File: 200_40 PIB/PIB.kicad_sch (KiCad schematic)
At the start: 34 parts, among them J1 Igniter, J10 TC2, J2 Rogowski, J3 PIB Interface, J6 Main Disch, J7 Heater 1, J8 Heater 1, J9 TC1, Q1 3300V, Q3 VO3120, Q8 IRF7403, Q9 IRF7403, U1 ACS37042KLHBLT-030B3, U10 TLP3543, U11 STM32G431KBTx, U14 VO618A, U3 BDJ2FC0WEFJ

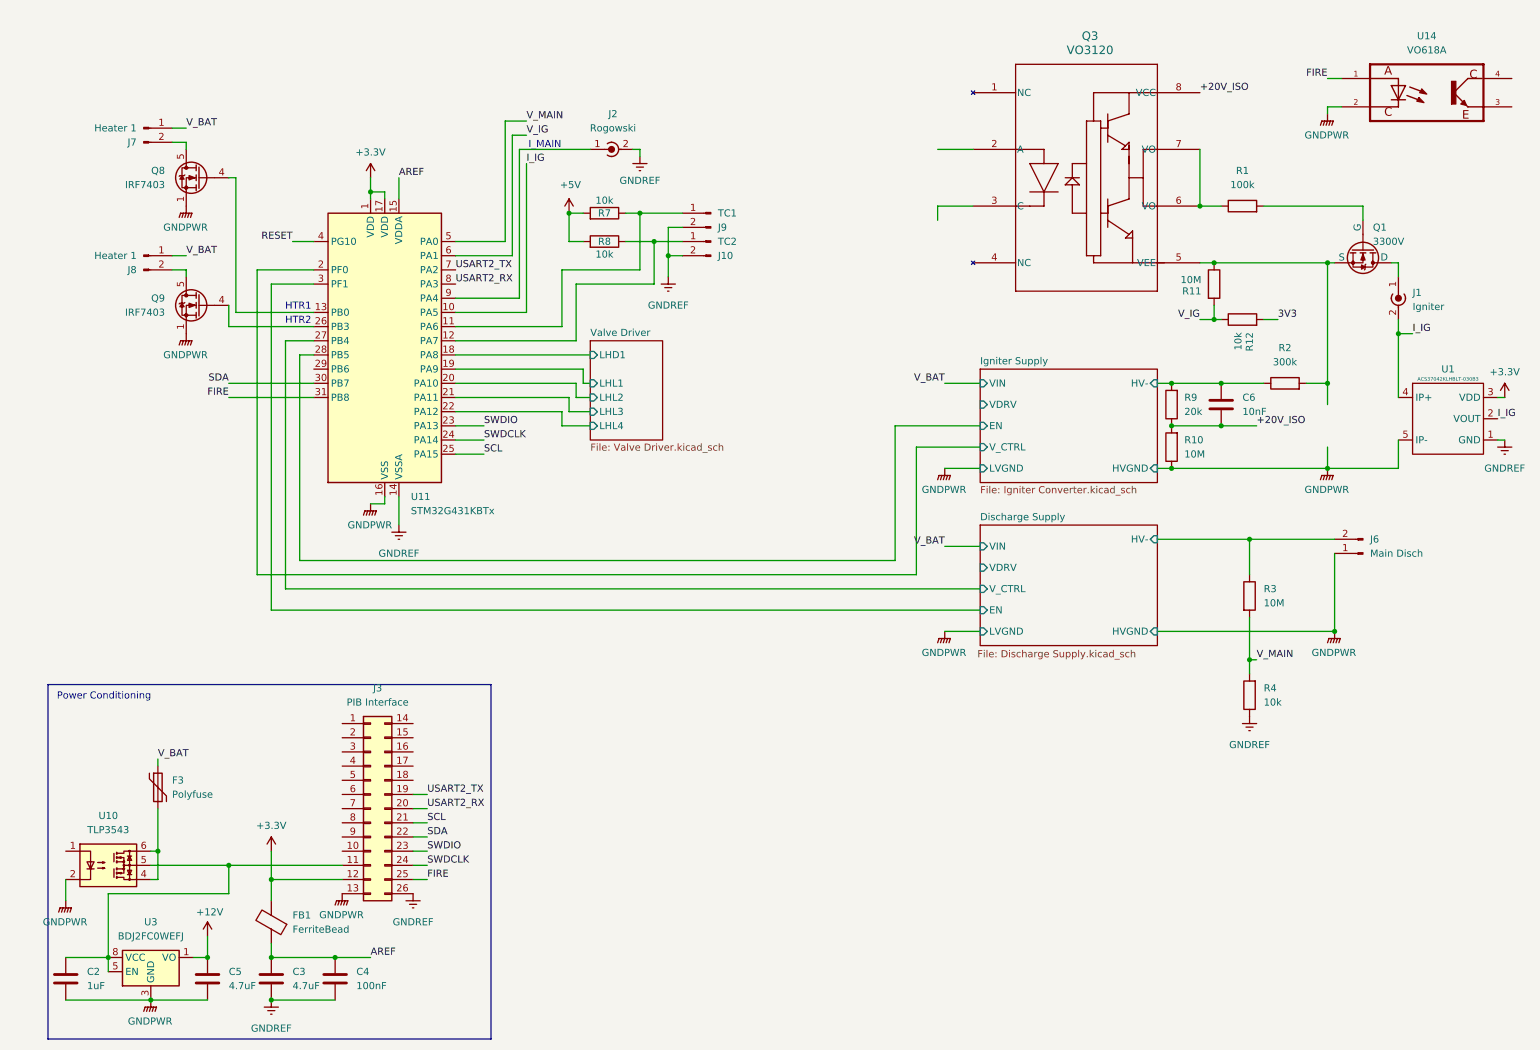
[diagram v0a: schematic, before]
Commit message: remove converters from PIB. WIP, do not check out
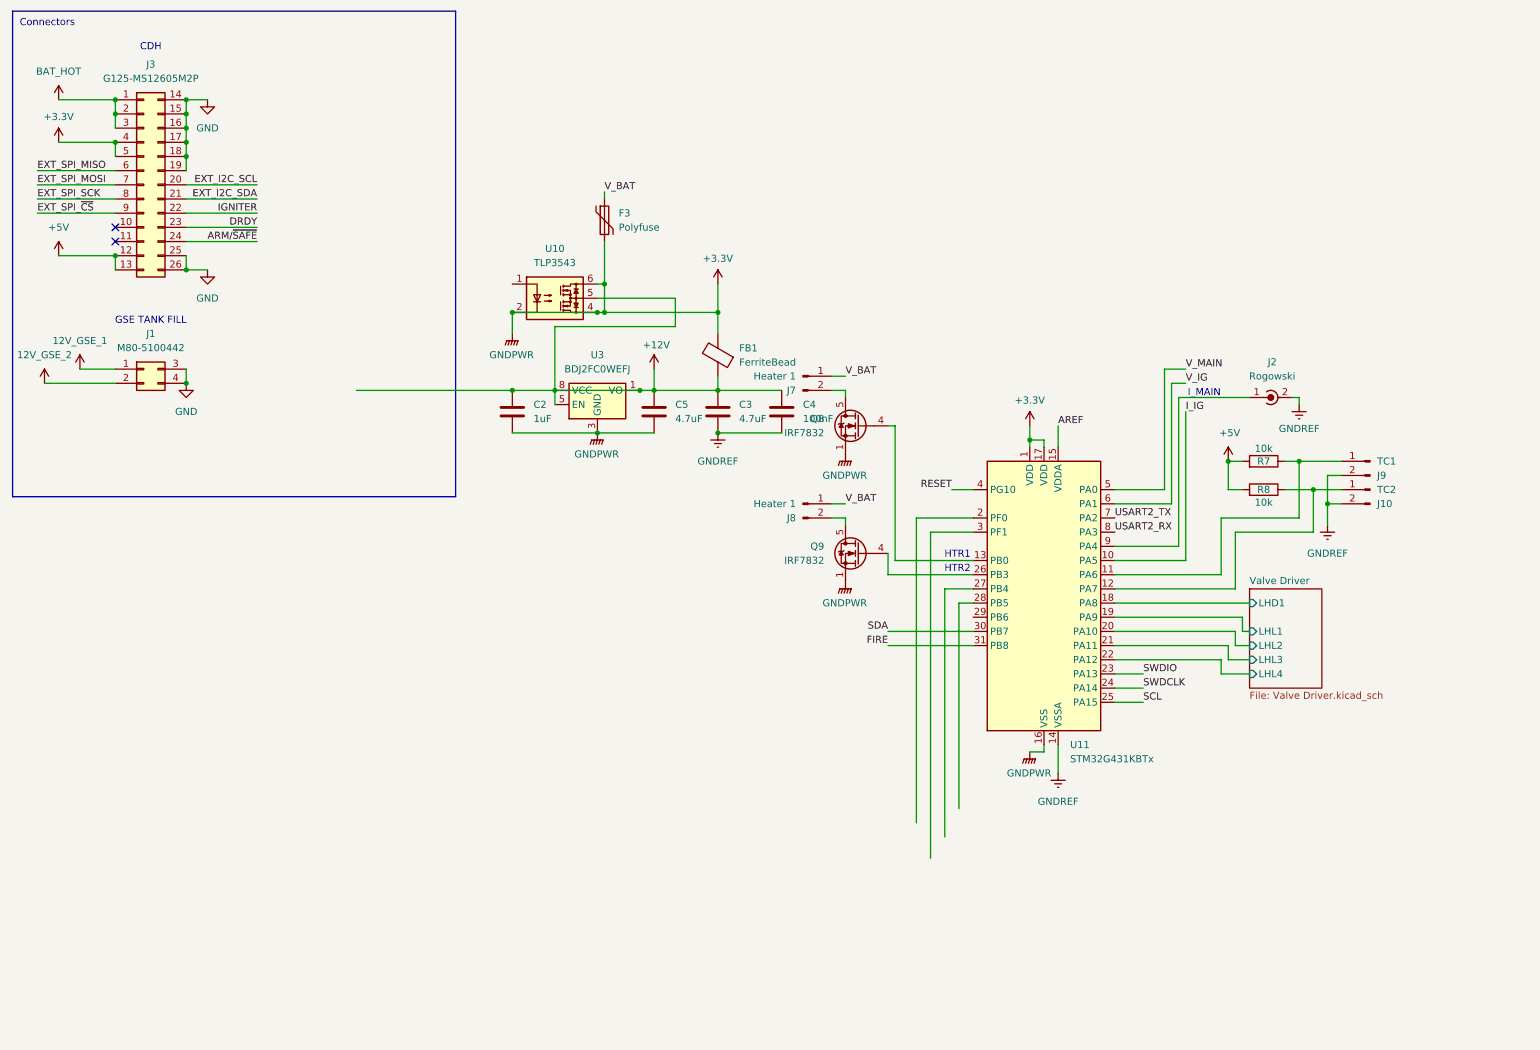
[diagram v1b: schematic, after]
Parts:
- removed C6: 10nF, symbol Device:C
- removed J1: Igniter, symbol Connector:Conn_Coaxial_Power
- removed J6: Main Disch, symbol Connector:Conn_01x02_Pin
- removed Q1: 3300V, Package_TO_SOT_THT:TO-247-4_Horizontal_TabDown, symbol Simulation_SPICE:NMOS
- removed Q3: VO3120, DIP_3120_VIS, symbol PIB_Symbol_Library:VO3120
- removed R1: 100k, symbol Device:R
- removed R10, R11, R3: 10M, symbol Device:R
- removed R12, R4: 10k, symbol Device:R
- removed R2: 300k, symbol Device:R
- removed R9: 20k, symbol Device:R
- removed U1: ACS37042KLHBLT-030B3, Package_TO_SOT_SMD:SOT-23-5_HandSoldering, symbol 0_PAY_Symbol_Library:ACS37042KLHBLT-030B3
- removed U14: VO618A, VO618A:DIP762W50P254L458H480Q4, symbol 0_PAY_Symbol_Library:VO618A
- added J1: M80-5100442, Package_LCC:PLCC-84_29.3x29.3mm_P1.27mm, symbol Connector_Generic:Conn_02x02_Top_Bottom
- J3: value PIB Interface -> G125-MS12605M2P
- Q8, Q9: value IRF7403 -> IRF7832
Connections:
- net +12V: now also C2.1, C3.1, C4.1, FB1.1, U10.5, U3.5 (EN), U3.8 (VCC)
- net +3.3V: now also C2.2, C5.2, F3.2, J3.4 (Pin_4), J3.5 (Pin_5), Q8.1 (S), Q8.2 (S), Q8.3 (S), Q9.1 (S), Q9.2 (S), Q9.3 (S), U10.2, U10.4, U10.6, U11.16 (VSS), U11.32 (VSS), U3.3 (GND), U3.9 (GND); no longer J3.12 (Pin_12)
- net +5V: now also J3.12 (Pin_12), J3.13 (Pin_13)
- net AREF: no longer C3.1, C4.1, FB1.1
- net FIRE: no longer J3.25 (Pin_25)
- net GNDREF: no longer J3.26 (Pin_26)
- net SCL: no longer J3.21 (Pin_21)
- net SDA: no longer J3.22 (Pin_22)
- net SWDCLK: no longer J3.24 (Pin_24)
- net SWDIO: no longer J3.23 (Pin_23)
- net USART2_RX: no longer J3.20 (Pin_20)
- net USART2_TX: no longer J3.19 (Pin_19)
- net BAT_HOT: now reaches J3.1 (Pin_1)
- net BAT_HOT: now also J3.2 (Pin_2), J3.3 (Pin_3)
- net GND: now reaches J3.14 (Pin_14)
- net GND: now also J3.15 (Pin_15), J3.16 (Pin_16), J3.17 (Pin_17), J3.18 (Pin_18), J3.19 (Pin_19), J3.25 (Pin_25), J3.26 (Pin_26), J1.3 (Pin_3), J1.4 (Pin_4)
- net EXT_SPI_MISO: now reaches J3.6 (Pin_6)
- net EXT_SPI_MOSI: now reaches J3.7 (Pin_7)
- net EXT_SPI_SCK: now reaches J3.8 (Pin_8)
- net EXT_SPI_~{CS}: now reaches J3.9 (Pin_9)
- net Discharge Supply/EN: no longer names the net of U11.3 (PF1)
- net Discharge Supply/V_CTRL: no longer names the net of U11.27 (PB4)
- removed net GNDPWR: C2.2, C5.2, J3.13 (Pin_13), Q8.1 (S), Q8.2 (S), Q8.3 (S), Q9.1 (S), Q9.2 (S), Q9.3 (S), U10.2, U11.16 (VSS), U11.32 (VSS), U3.3 (GND), U3.9 (GND)
- net Igniter Supply/EN: no longer names the net of U11.28 (PB5)
- net Igniter Supply/V_CTRL: no longer names the net of U11.2 (PF0)
- new net 12V_GSE_1: J1.1 (Pin_1)
- new net 12V_GSE_2: J1.2 (Pin_2)
- new net ARM/~{SAFE}: J3.24 (Pin_24)
- new net DRDY: J3.23 (Pin_23)
- new net EXT_I2C_SCL: J3.20 (Pin_20)
- new net EXT_I2C_SDA: J3.21 (Pin_21)
- new net IGNITER: J3.22 (Pin_22)
- now unconnected: J3.11 (Pin_11)
- no-connect marks 0 -> 2
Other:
- removed sheet Discharge Supply
- removed sheet Igniter Supply
- note added: "CDH"
- note added: "Connectors"
- note added: "GSE TANK FILL"
- note removed: "Power Conditioning"
- moved on the sheet: C2, C3, C4, C5, F3, FB1, J10, J2, J3, J7, J8, J9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
